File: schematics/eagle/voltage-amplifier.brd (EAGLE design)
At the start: 31.7 x 28.1 mm, 15 parts, among them Q1 2N3904, Q2 2N3904, Q3 2N3904, Q4 2N3904

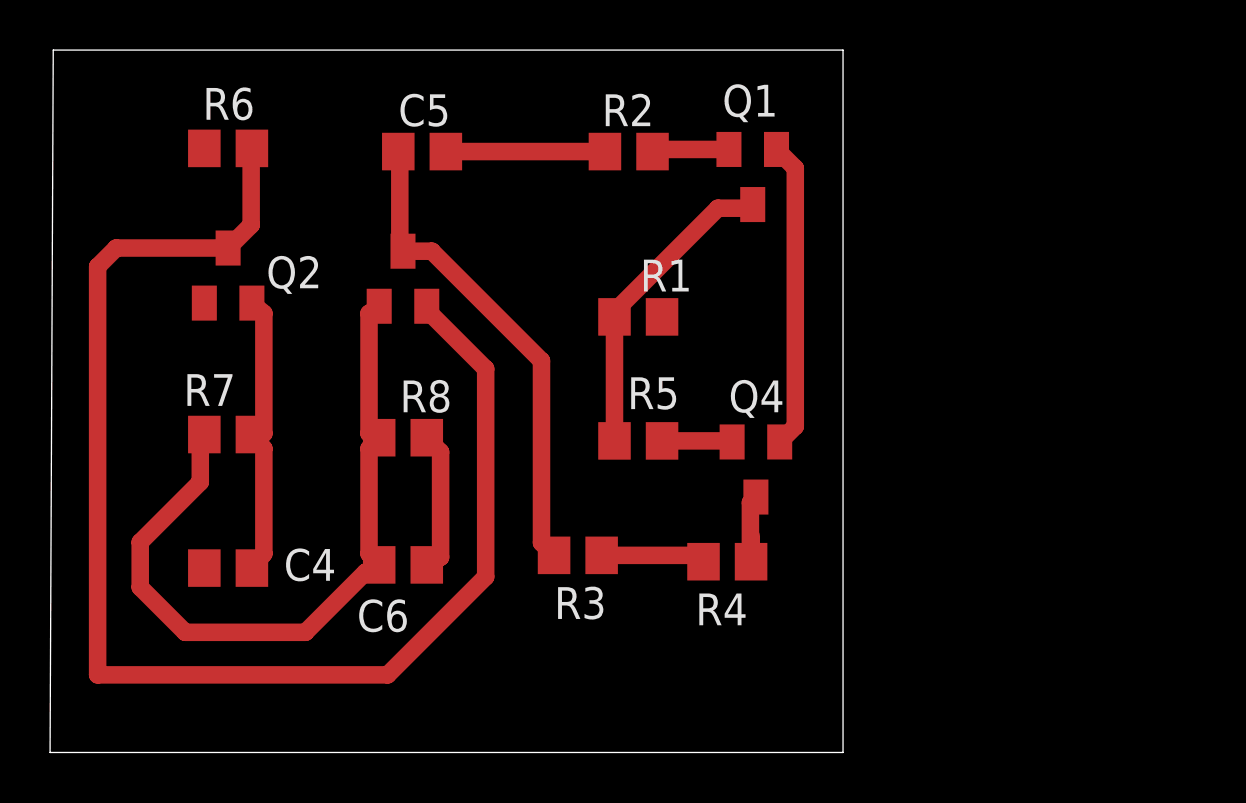
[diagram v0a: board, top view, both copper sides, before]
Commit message: Voltage Amplifier PCB
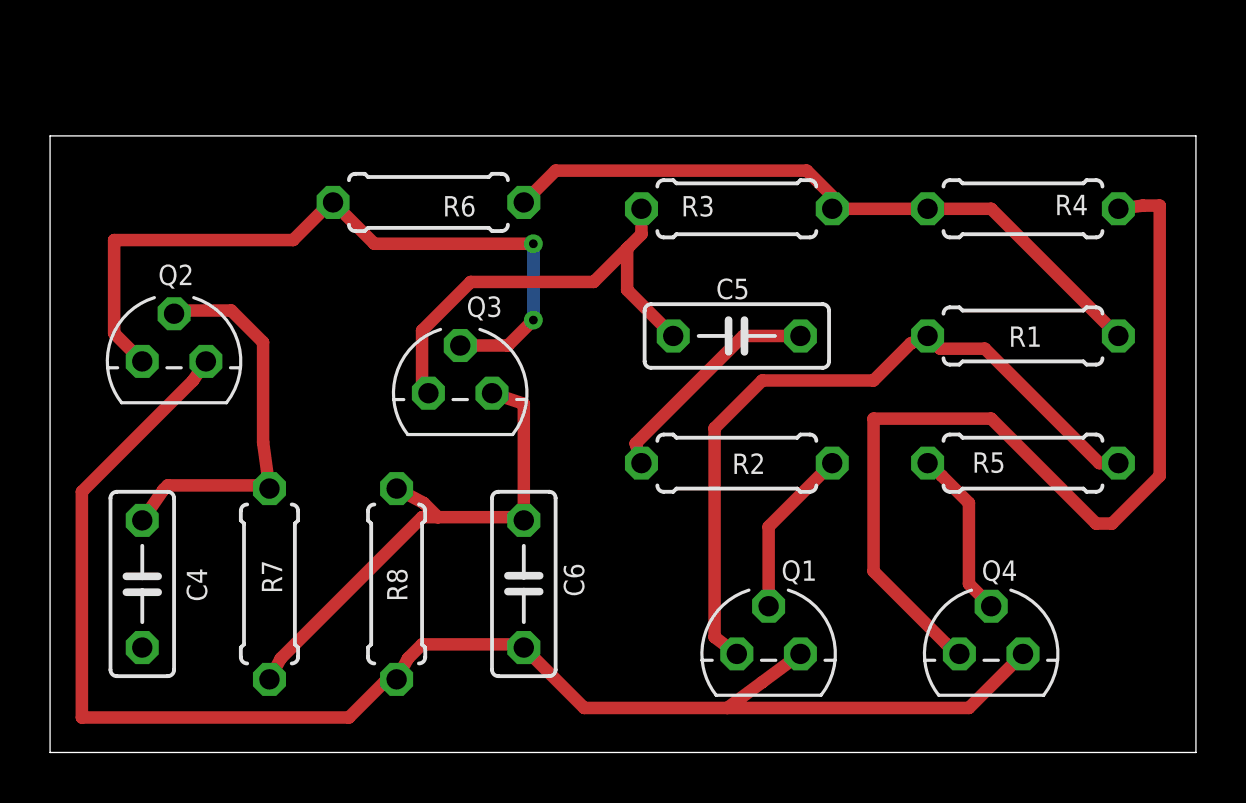
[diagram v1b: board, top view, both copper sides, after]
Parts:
- C4, C5, C6: device sym:C0805 -> sym-toh:C050-025X075
- Q1, Q2, Q3, Q4: device sym:SOT23 -> sym-toh:TO92
- R1, R2, R3, R4, R5, R6, R7, R8: device sym:R0805 -> sym-toh:0207/7
- moved Q1 19.1 mm to (28.7, 3.94), turned to 0 degrees
- moved R4 18.4 mm to (38.9, 21.7)
- moved R5 15.4 mm to (38.9, 11.6), turned to 0 degrees
- moved R1 15.4 mm to (38.9, 16.6)
- moved R3 15.2 mm to (27.4, 21.7)
- moved C5 14.6 mm to (27.4, 16.6)
- moved R2 13.2 mm to (27.4, 11.6)
- moved Q4 11.9 mm to (37.6, 3.94), turned to 0 degrees
- moved R6 8.29 mm to (15.1, 22.0), turned to 180 degrees
- moved R7 6.19 mm to (8.76, 6.73), turned to 90 degrees
- moved R8 5.85 mm to (13.8, 6.73), turned to 270 degrees
- moved Q3 5.11 mm to (16.4, 14.4)
- moved C6 4.89 mm to (18.9, 6.73), turned to 90 degrees
- moved Q2 4.05 mm to (4.95, 15.6)
- moved C4 3.49 mm to (3.68, 6.73), turned to 270 degrees
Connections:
- removed net N$4: R1.1
- removed net N$9: R6.1
- net V+: now also R1.1, R6.1
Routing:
- net 0: track 17.9 -> 60.8 mm
- net VOUT: track 4.19 -> 37.3 mm
- net N$8: track 55.1 -> 30.1 mm, vias 0 -> 2
- net V+: track 4.17 -> 27.5 mm
- net N$3: track 12.5 -> 29.2 mm
- net N$11: track 29.7 -> 21.1 mm
- net N$10: track 11.6 -> 15.9 mm
- net N$1: track 2.82 -> 6.79 mm
- net N$7: track 3.09 -> 6.77 mm
- net N$6: track 6.36 -> 9.18 mm
- net N$5: track 19.4 -> 18.7 mm
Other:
- board size 31.7 x 28.1 mm -> 45.8 x 24.6 mm
